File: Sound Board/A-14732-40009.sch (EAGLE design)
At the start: 206 parts, among them IC1 74LS374DW, P2 AUX IN, P3 AUX OUT, P4 ORKIN R/W, P5 VOLUME, Q1 MPS3646, U1 OKI6295, U11 26LS32A, U12 27C040-150, U13 27C040-150, U14 YAMAHA 2151, U15 TIL7524, U16 74LS374, U17 74LS174, U18 16L8, U19 74LS11, U2 2064, U20 74LS139, U21 74LS14, U22 74LS74, U23 74LS74, U24 26LS32A, U25 26LS32A, U26 74LS04, U28 YAMAHA 3012, U29 LM324D, U3 27C040, U30 MC3340, U31 HA3116, U32 TL084D, U33 TL084D, U4 6809E, U5 26LS31, U6 26LS31, U7 26LS31, U8 74LS138, U9 74LS74, Y1 3.5749MHz, Y2 8MHz

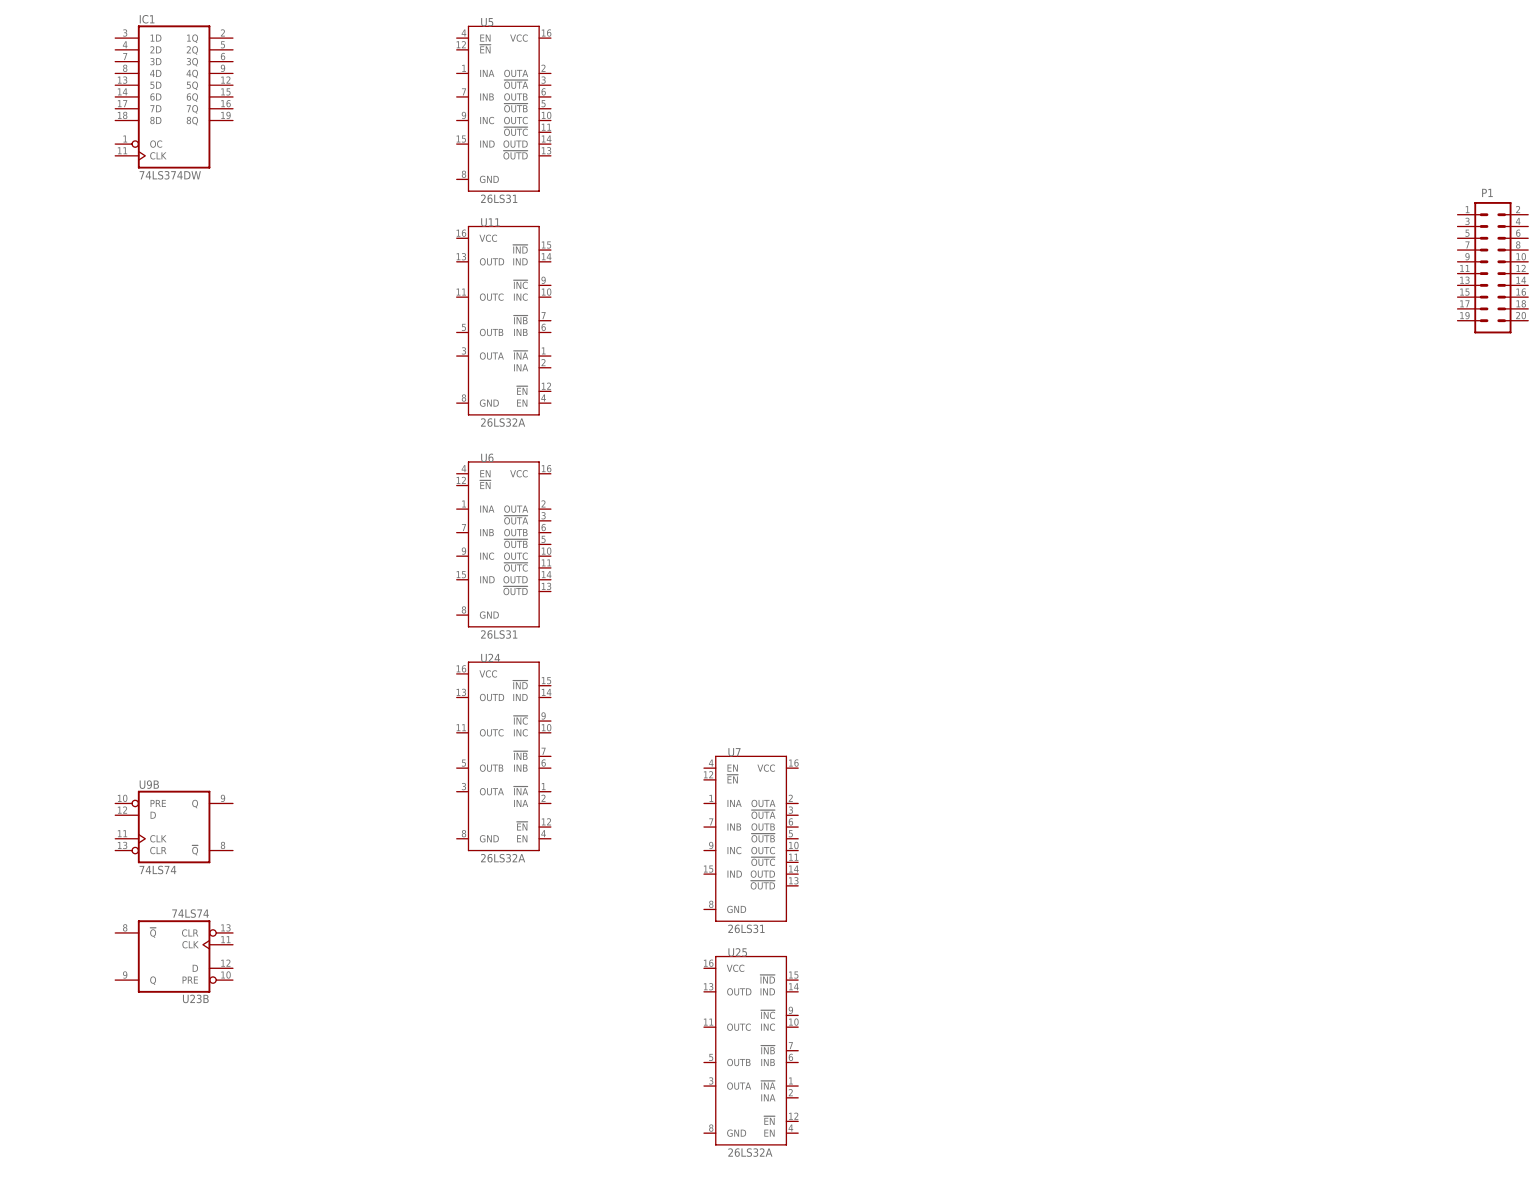
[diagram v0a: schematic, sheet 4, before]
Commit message: wip
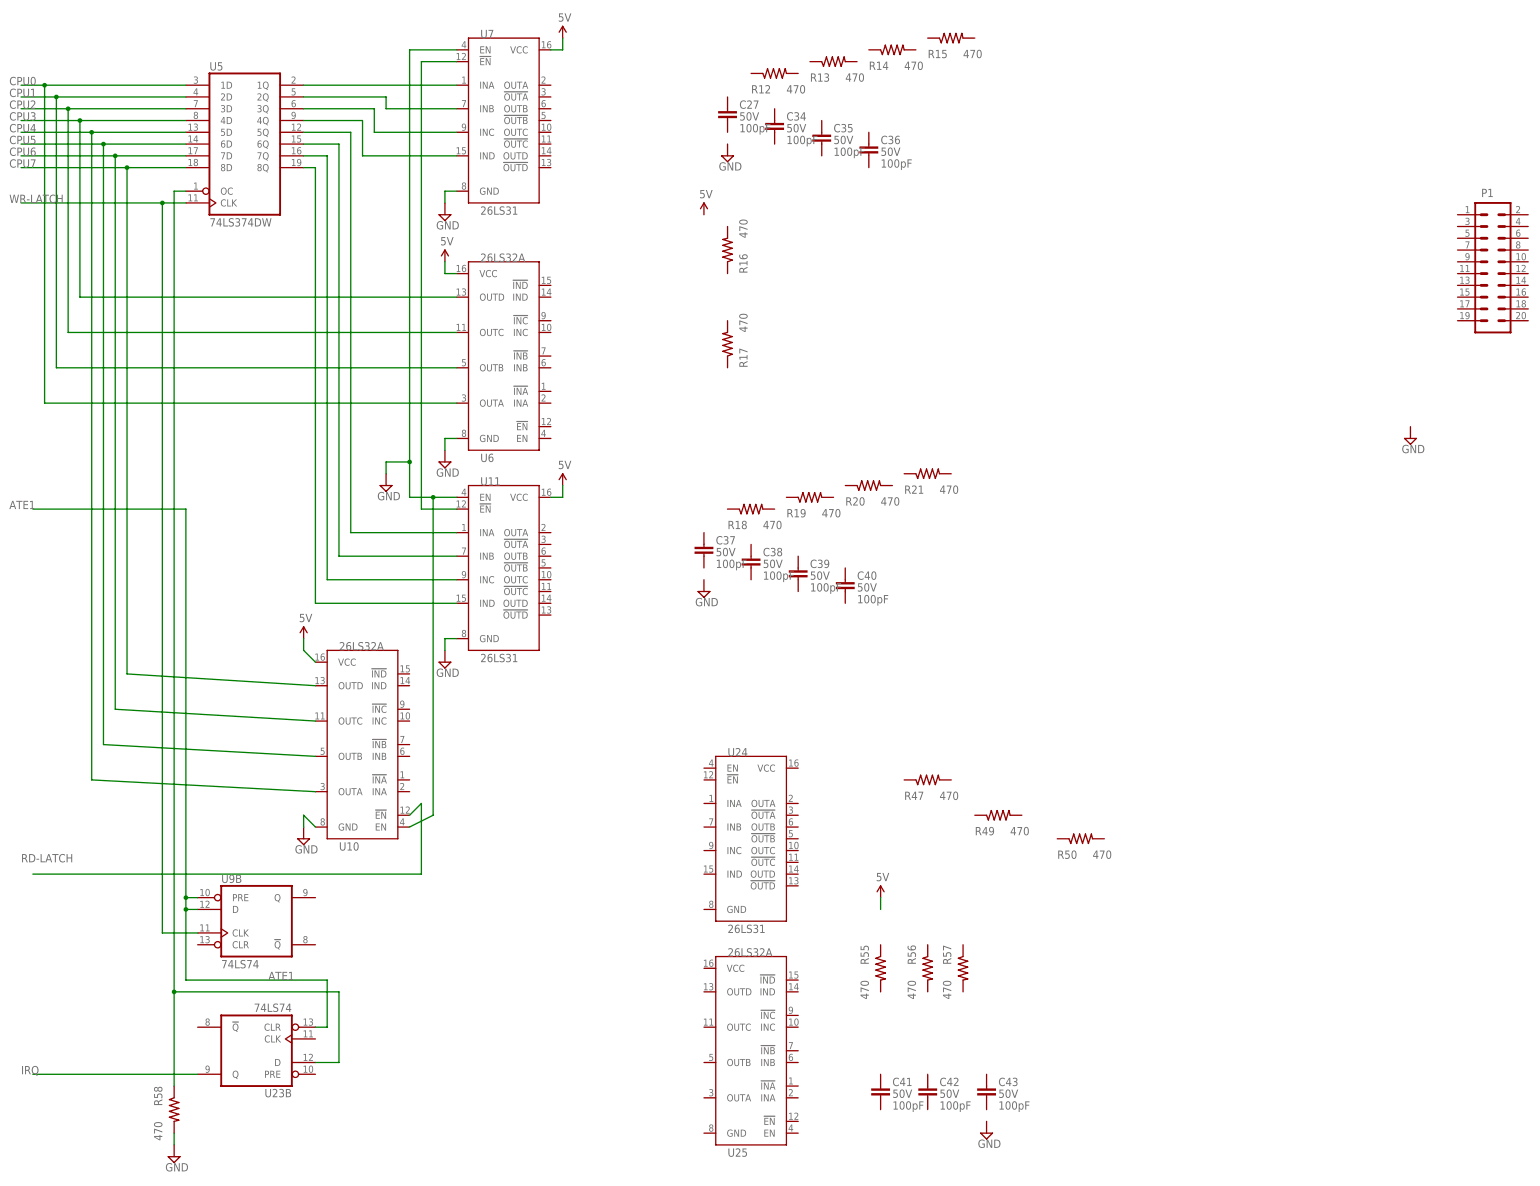
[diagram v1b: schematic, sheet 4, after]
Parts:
- removed IC1: 74LS374DW, 74xx-us:74LS374DW
- added C27, C34, C35, C36, C37, C38, C39, C40, C41, C42, C43: 100pF, SparkFun-Capacitors:1.0UF50V10%(1206)
- added R12, R13, R14, R15, R16, R17, R18, R19, R20, R21, R47, R49, R50, R55, R56, R57, R58: 470, resistor:R-US_R1206
- added U10: 26LS32A, A-14732-40009:26LS32A
- U11, U24: value 26LS32A -> 26LS31; device A-14732-40009:26LS32A -> A-14732-40009:26LS31
- U5: value 26LS31 -> 74LS374DW; device A-14732-40009:26LS31 -> 74xx-us:74LS374DW
- U6: value 26LS31 -> 26LS32A; device A-14732-40009:26LS31 -> A-14732-40009:26LS32A
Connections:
- new net N$104: U5A.2Q, U7.INB
- new net N$105: U5A.3Q, U7.INC
- new net N$106: U5A.4Q, U7.IND
- new net N$107: U11.INA, U5A.5Q
- new net N$108: U11.INB, U5A.6Q
- new net N$109: U11.INC, U5A.7Q
- new net N$110: U11.IND, U5A.8Q
- new net N$111: U11.!EN, U7.!EN
- new net N$112: R58.1, U23B.D, U5A.OC
- new net N$98: U5A.1Q, U7.INA
- net 5V: now also U10.VCC, U11.VCC, U6.VCC, U7.VCC
- net ATE1: now also U23B.CLR, U9B.D, U9B.PRE
- net CPU0: now also U5A.1D, U6.OUTA
- net CPU1: now also U5A.2D, U6.OUTB
- net CPU2: now also U5A.3D, U6.OUTC
- net CPU3: now also U5A.4D, U6.OUTD
- net CPU4: now also U10.OUTA, U5A.5D
- net CPU5: now also U10.OUTB, U5A.6D
- net CPU6: now also U10.OUTC, U5A.7D
- net CPU7: now also U10.OUTD, U5A.8D
- net GND: now also R58.2, U10.EN, U10.GND, U11.EN, U11.GND, U6.GND, U7.EN, U7.GND
- net IRQ: now also U23B.Q
- net RD-LATCH: now also U10.!EN
- net WR-LATCH: now also U5A.CLK, U9B.CLK
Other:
- moved on the sheet: U11, U23B, U24, U6, U7, U9B
